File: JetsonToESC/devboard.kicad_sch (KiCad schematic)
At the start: 14 parts, among them U1 ESP32-C3_SUPERMINI_TH, U4 MCP23018x-x-SS, U6 ULN2003

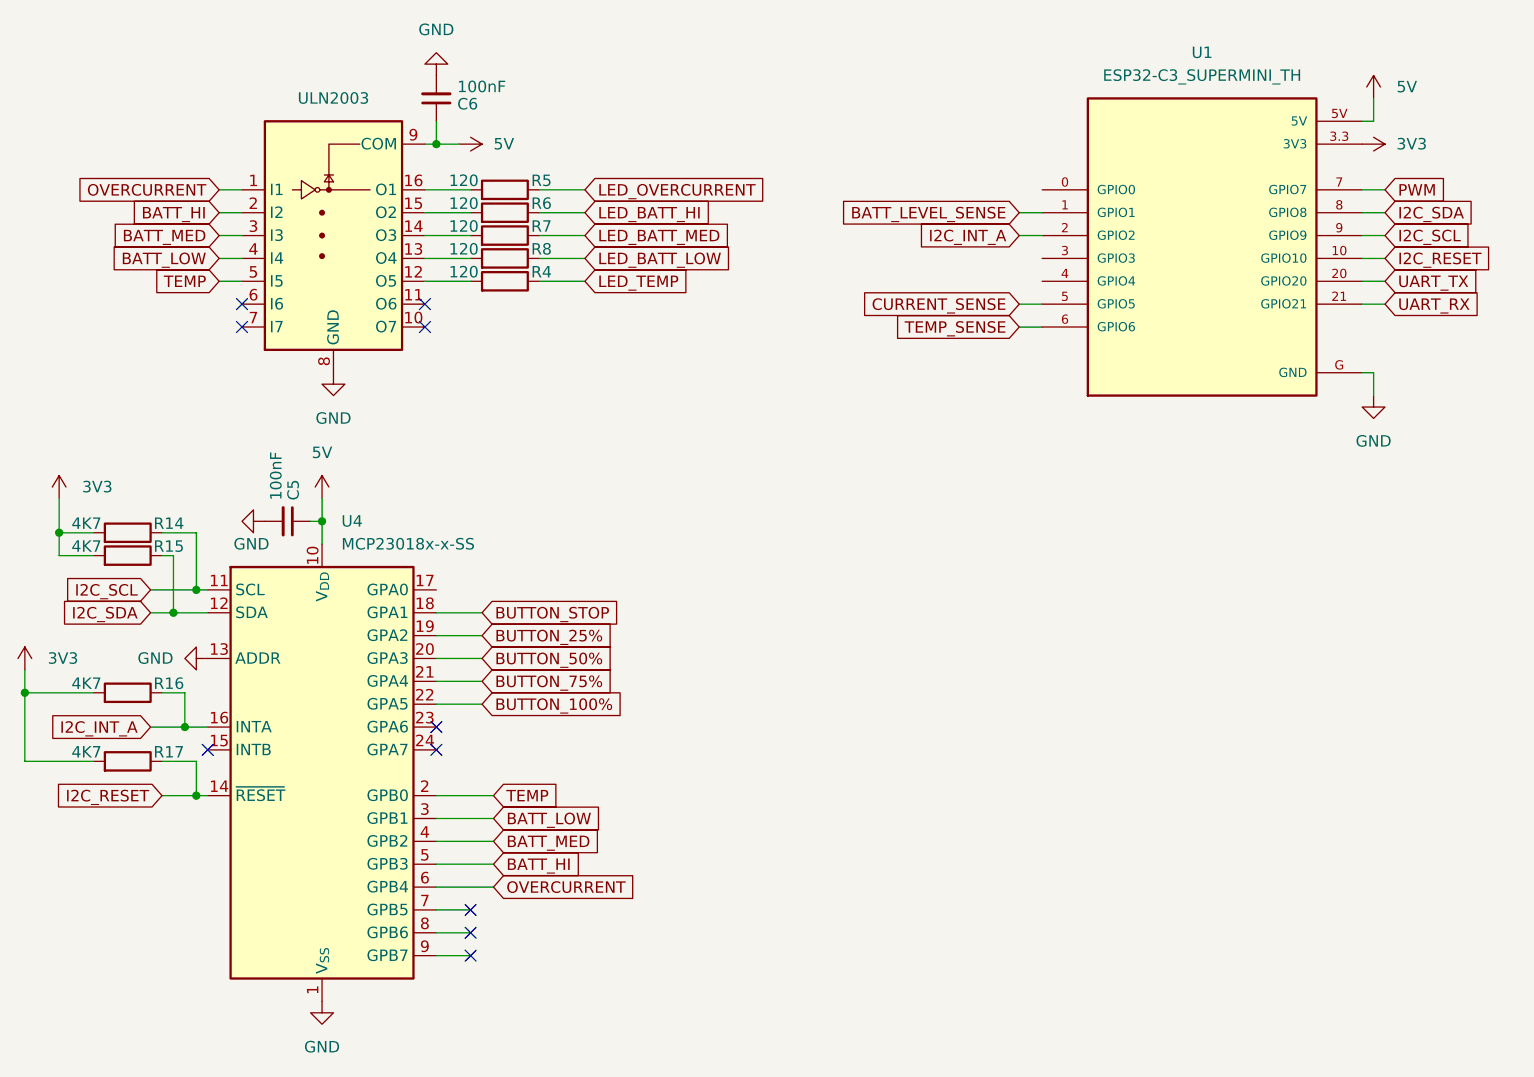
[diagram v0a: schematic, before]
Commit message: Updated for v2.0, almost complete
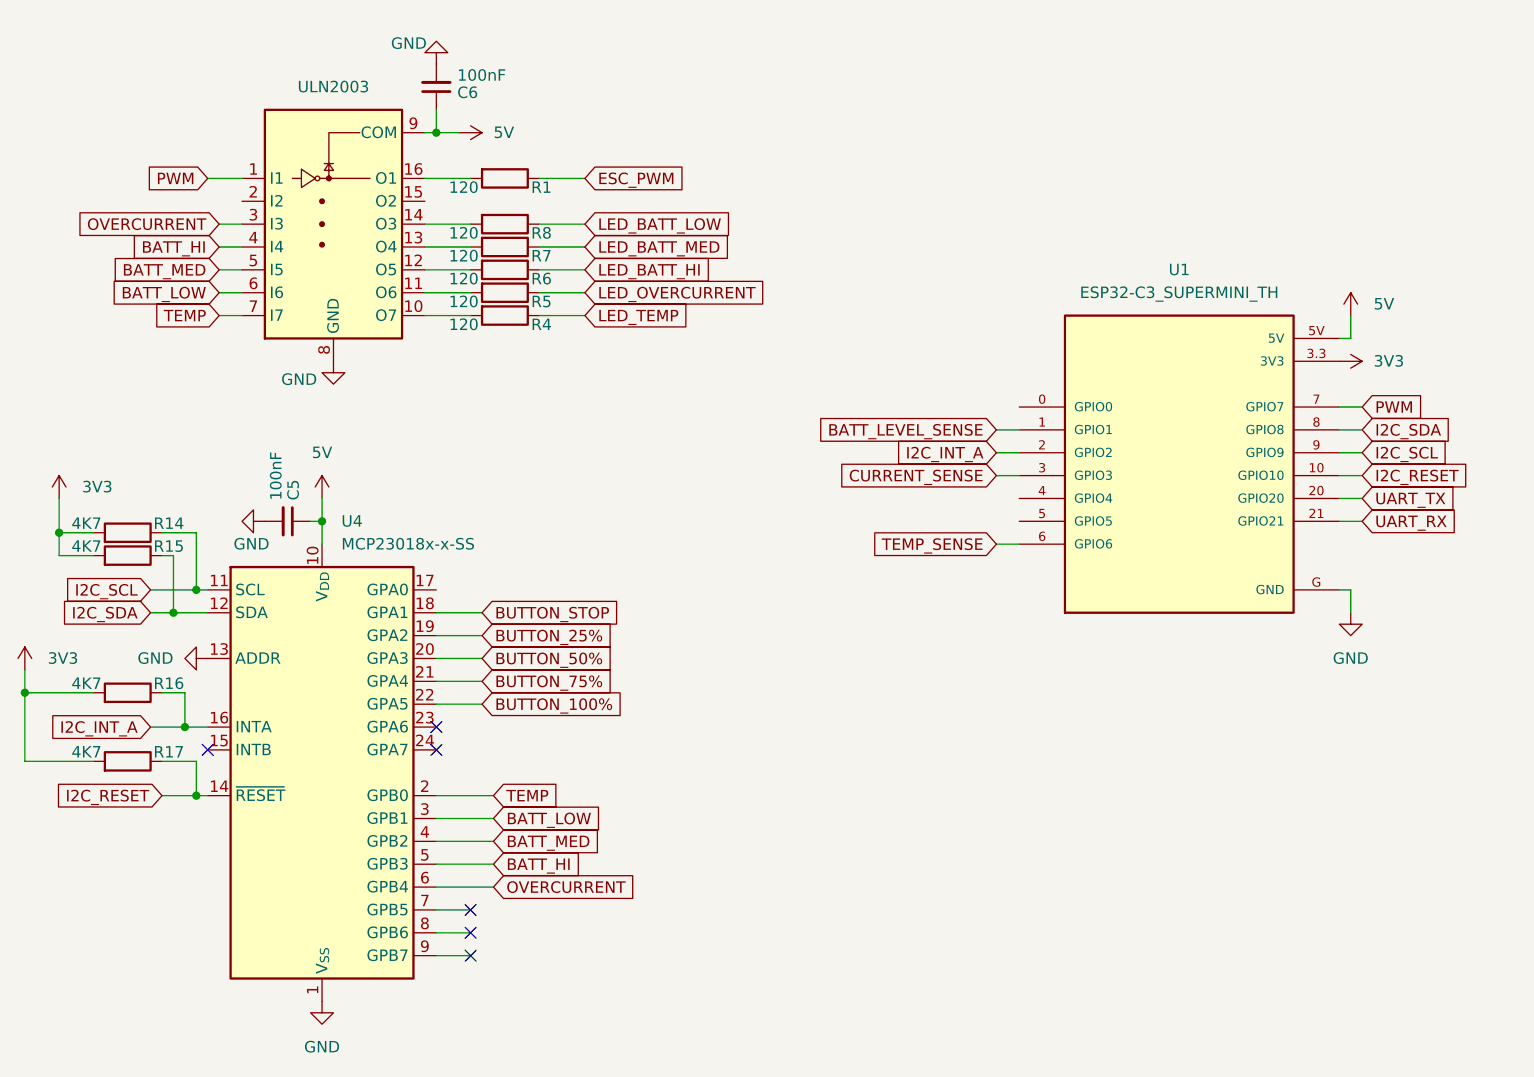
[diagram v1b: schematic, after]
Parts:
- added R1: 120, Resistor_SMD:R_0603_1608Metric, symbol Device:R
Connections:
- net BATT_HI: now also U6.4 (I4); no longer U6.2 (I2)
- net BATT_LOW: now also U6.6 (I6); no longer U6.4 (I4)
- net BATT_MED: now also U6.5 (I5); no longer U6.3 (I3)
- net CURRENT_SENSE: now also U1.3 (GPIO3); no longer U1.5 (GPIO5)
- net OVERCURRENT: now also U6.3 (I3); no longer U6.1 (I1)
- net PWM: now also U6.1 (I1)
- net TEMP: now also U6.7 (I7); no longer U6.5 (I5)
- net at R6.2: now also U6.12 (O5); no longer U6.15 (O2)
- net at R7.2: now also U6.13 (O4); no longer U6.14 (O3)
- net at R5.2: now also U6.11 (O6); no longer U6.16 (O1)
- net at R8.2: now also U6.14 (O3); no longer U6.13 (O4)
- net at U6.10 (O7): now also R4.2
- new net: R1.2, U6.16 (O1)
- new net ESC_PWM: R1.1
- no-connect marks 10 -> 6
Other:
- moved on the sheet: C6, R4, R5, R6, R7, R8, U1
